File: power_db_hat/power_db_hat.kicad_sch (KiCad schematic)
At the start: 82 parts, among them J2 BAT1, J3 12V_out, J4 Conn_01x04_Pin, J5 24V_out, J6 PD_power, J7 Conn_01x20_Pin, J8 BAT2

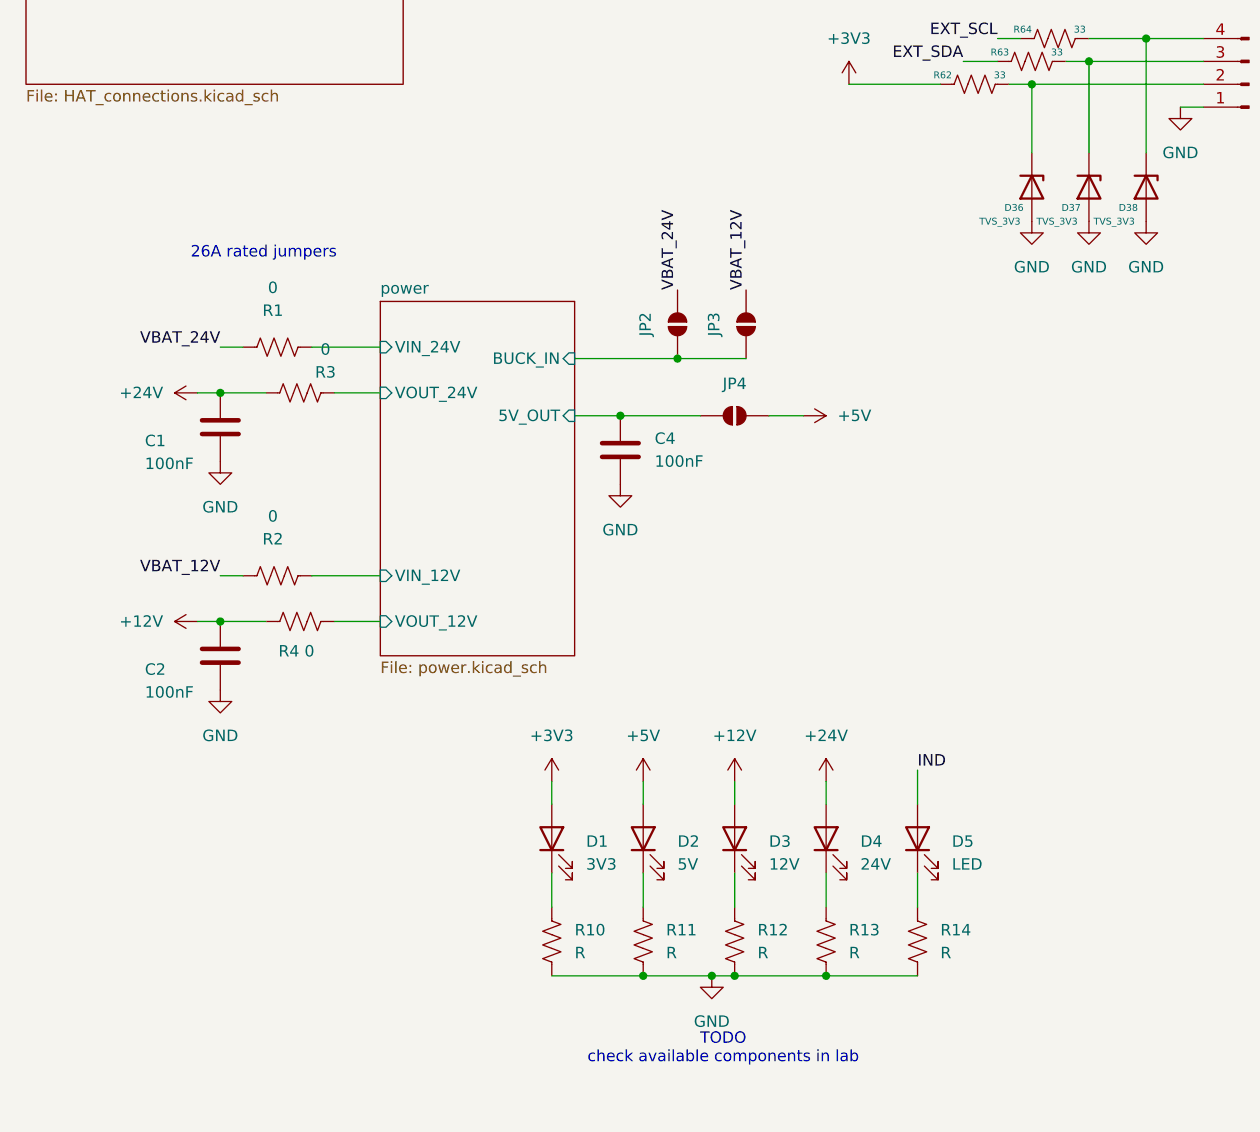
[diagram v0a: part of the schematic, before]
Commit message: lol
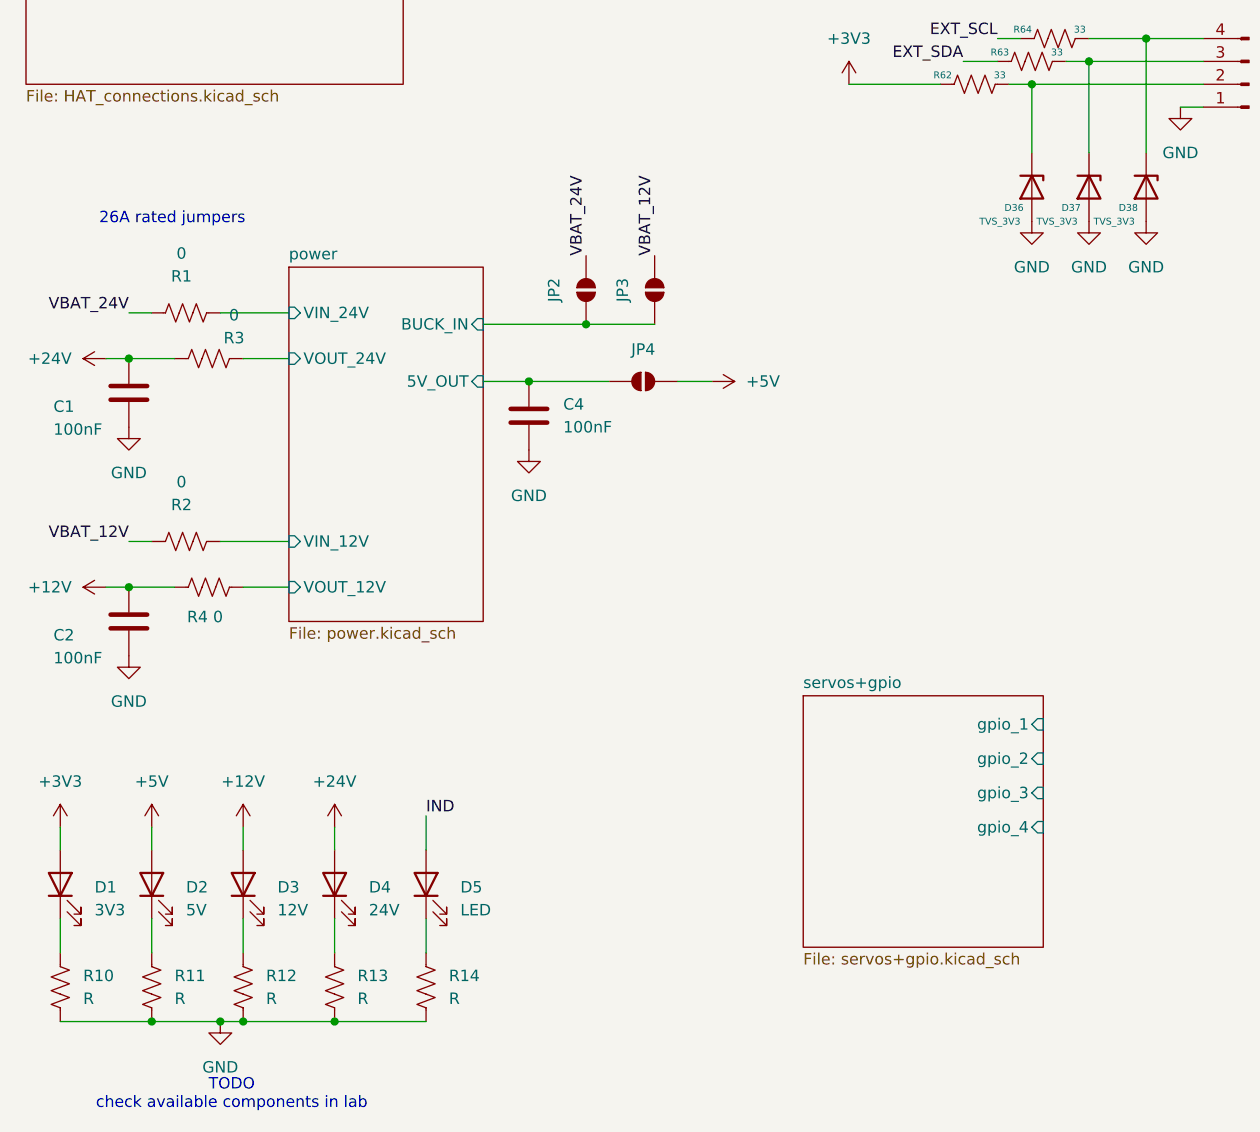
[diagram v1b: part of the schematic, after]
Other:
- added sheet servos+gpio (servos+gpio.kicad_sch)
- moved on the sheet: C1, C2, C4, D1, D2, D3, D4, D5, JP2, JP3, JP4, R1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
